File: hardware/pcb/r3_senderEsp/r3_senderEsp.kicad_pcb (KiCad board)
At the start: 2 copper layers, 165.5 x 125.5 mm, 17 parts, among them J1 RFID-RC522, J2 KY-021, J3 KY-021, J4 Links, J5 Rechts

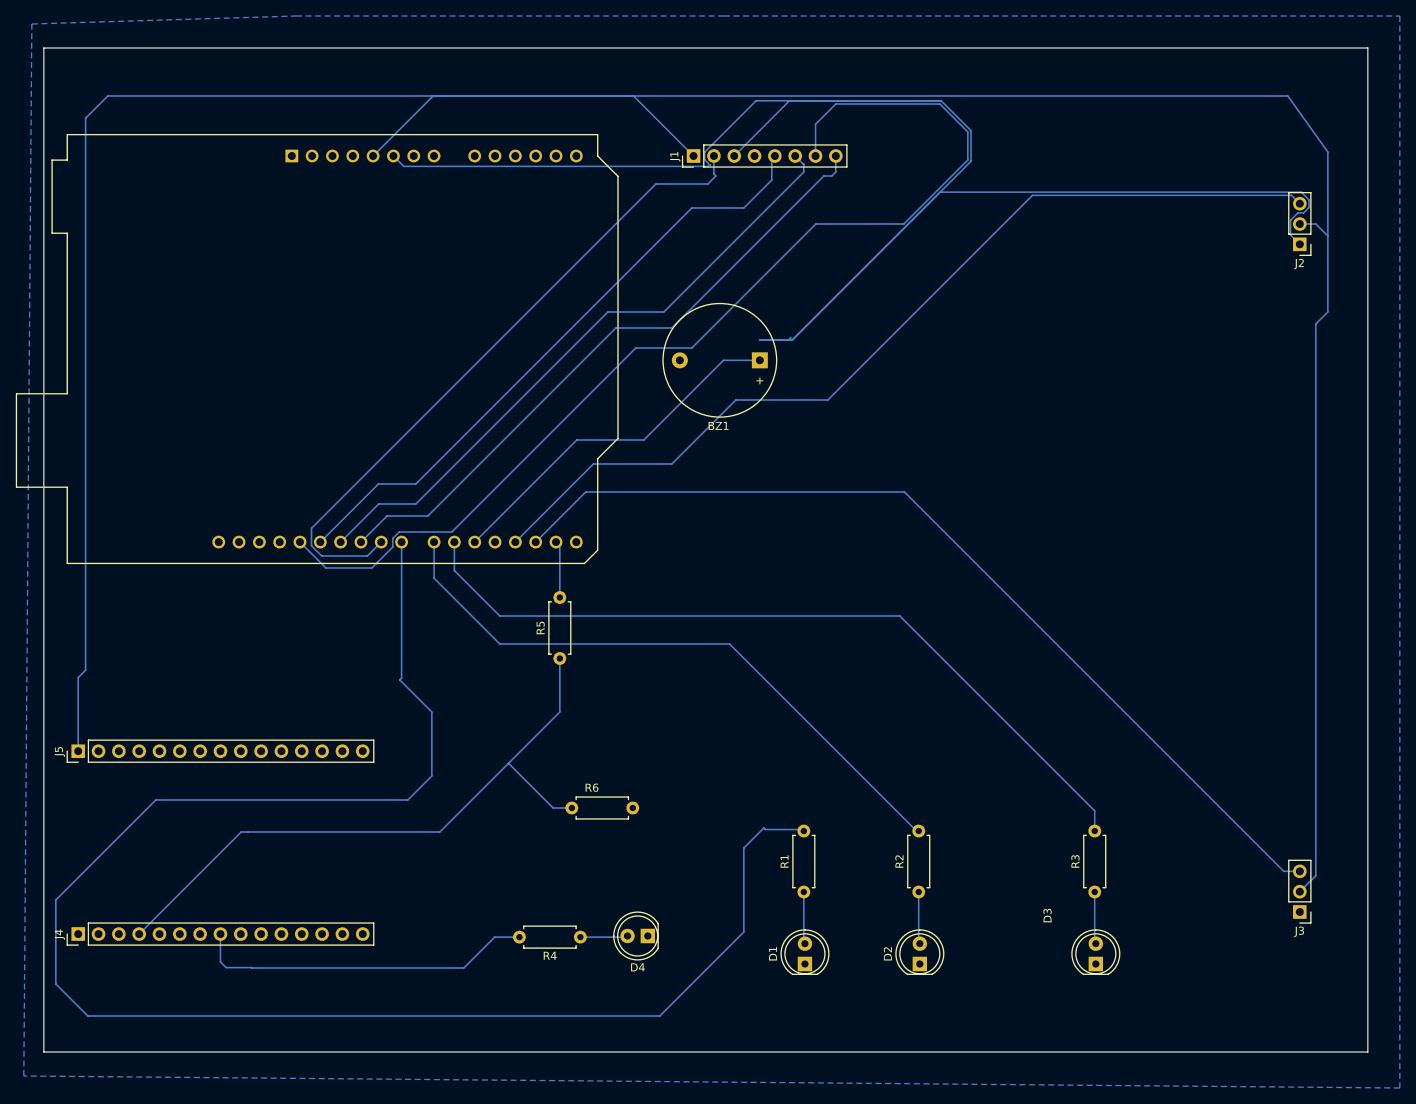
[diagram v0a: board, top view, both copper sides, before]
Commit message: Add files via upload
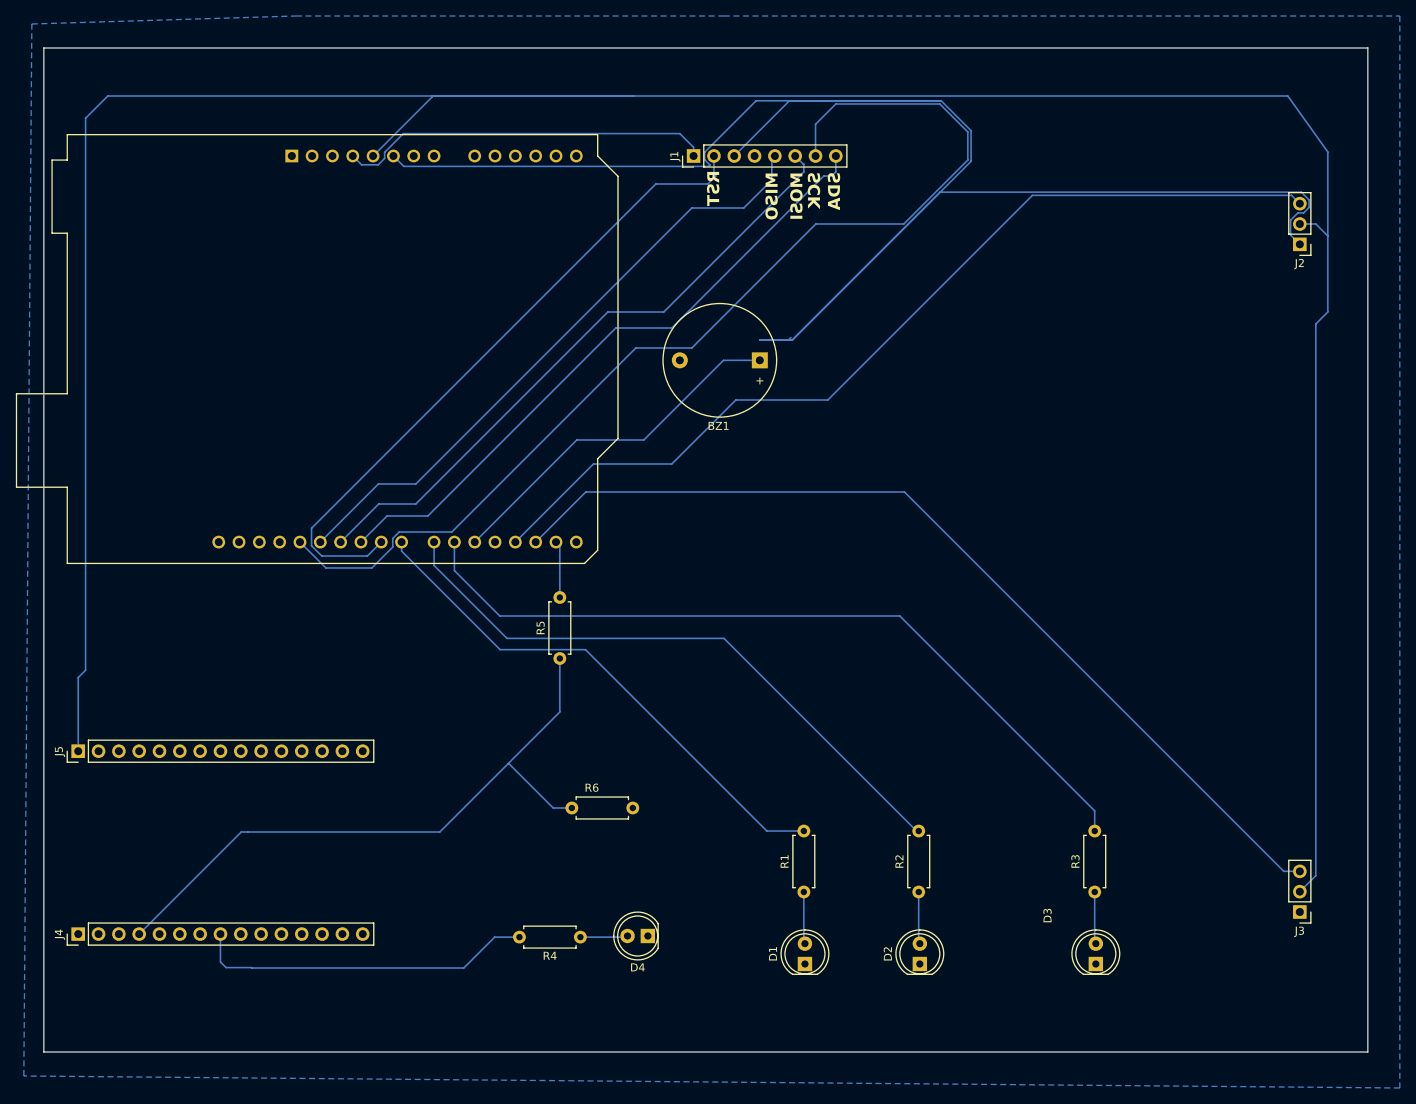
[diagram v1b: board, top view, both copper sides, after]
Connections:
- A1 pad 4: unconnected-(A1-3V3-Pad4) -> Net-(A1-3V3)
- J1 pad 1: +5V -> Net-(A1-3V3)
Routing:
- net Net-(A1-D8): track 206.0 -> 65.9 mm
- net Net-(A1-3V3): track 0.00 -> 46.9 mm
- net +5V: track 257.8 -> 247.2 mm
- net Net-(A1-D7): track 78.3 -> 77.4 mm
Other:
- board text added: "MISO"
- board text added: "MOSI"
- board text added: "RST"
- board text added: "SCK"
- board text added: "SDA"
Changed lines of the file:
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@@
 			(drillshape 0)
 			(scaleselection 1)
-			(outputdirectory "Kicad Datein/GerberBohrungen/")
+			(outputdirectory "r3_senderEsp_GerberBohrungen")
 		)
 	)
@@
 	(net 1 "Net-(A1-D2)")
 	(net 2 "unconnected-(A1-A2-Pad11)")
-	(net 3 "unconnected-(A1-3V3-Pad4)")
+	(net 3 "Net-(A1-3V3)")
 	(net 4 "Net-(A1-D13)")
 	(net 5 "unconnected-(A1-D0{slash}RX-Pad15)")
@@
 		(property ki_fp_filters "LED* LED_SMD:* LED_THT:*")
 		(sheetname "/")
-		(sheetfile "R3Sender.kicad_sch")
+		(sheetfile "r3_senderEsp.kicad_sch")
 		(attr through_hole)
 		(fp_line
@@
 		(property ki_fp_filters "Connector*:*_1x??_*")
 		(sheetname "/")
-		(sheetfile "R3Sender.kicad_sch")
+		(sheetfile "r3_senderEsp.kicad_sch")
 		(attr through_hole)
 		(fp_line
@@
 			(layers "*.Cu" "*.Mask")
 			(remove_unused_layers no)
-			(net 10 "+5V")
+			(net 3 "Net-(A1-3V3)")
 			(pinfunction "Pin_1")
 			(pintype "passive")
@@
 		(property ki_fp_filters "Connector*:*_1x??_*")
 		(sheetname "/")
-		(sheetfile "R3Sender.kicad_sch")
+		(sheetfile "r3_senderEsp.kicad_sch")
 		(attr through_hole)
 		(fp_line
@@
 		(property ki_fp_filters "R_*")
 		(sheetname "/")
-		(sheetfile "R3Sender.kicad_sch")
+		(sheetfile "r3_senderEsp.kicad_sch")
 		(attr through_hole)
 		(fp_line
@@
 		(property ki_fp_filters "R_*")
 		(sheetname "/")
-		(sheetfile "R3Sender.kicad_sch")
+		(sheetfile "r3_senderEsp.kicad_sch")
 		(attr through_hole)
 		(fp_line
@@
 		(property ki_fp_filters "Arduino*UNO*R3*")
 		(sheetname "/")
-		(sheetfile "R3Sender.kicad_sch")
+		(sheetfile "r3_senderEsp.kicad_sch")
 		(attr through_hole)
 		(fp_line
@@
 			(layers "*.Cu" "*.Mask")
 			(remove_unused_layers no)
-			(net 3 "unconnected-(A1-3V3-Pad4)")
+			(net 3 "Net-(A1-3V3)")
 			(pinfunction "3V3")
 			(pintype "power_out")
@@
 		(property ki_fp_filters "LED* LED_SMD:* LED_THT:*")
 		(sheetname "/")
-		(sheetfile "R3Sender.kicad_sch")
+		(sheetfile "r3_senderEsp.kicad_sch")
 		(attr through_hole)
 		(fp_line
@@
 		(property ki_fp_filters "LED* LED_SMD:* LED_THT:*")
 		(sheetname "/")
-		(sheetfile "R3Sender.kicad_sch")
+		(sheetfile "r3_senderEsp.kicad_sch")
 		(attr through_hole)
 		(fp_line
@@
 		(property ki_fp_filters "R_*")
 		(sheetname "/")
-		(sheetfile "R3Sender.kicad_sch")
+		(sheetfile "r3_senderEsp.kicad_sch")
 		(attr through_hole)
 		(fp_line
@@
 		(property ki_fp_filters "Connector*:*_1x??_*")
 		(sheetname "/")
-		(sheetfile "R3Sender.kicad_sch")
+		(sheetfile "r3_senderEsp.kicad_sch")
 		(attr through_hole)
 		(fp_line
@@
 		(property ki_fp_filters "R_*")
 		(sheetname "/")
-		(sheetfile "R3Sender.kicad_sch")
+		(sheetfile "r3_senderEsp.kicad_sch")
 		(attr through_hole)
 		(fp_line
@@
 		(property ki_fp_filters "LED* LED_SMD:* LED_THT:*")
 		(sheetname "/")
-		(sheetfile "R3Sender.kicad_sch")
+		(sheetfile "r3_senderEsp.kicad_sch")
 		(attr through_hole)
 		(fp_line
@@
 		(property ki_fp_filters "R_*")
 		(sheetname "/")
-		(sheetfile "R3Sender.kicad_sch")
+		(sheetfile "r3_senderEsp.kicad_sch")
 		(attr through_hole)
 		(fp_line
@@
 		(property ki_fp_filters "Connector*:*_1x??_*")
 		(sheetname "/")
-		(sheetfile "R3Sender.kicad_sch")
+		(sheetfile "r3_senderEsp.kicad_sch")
 		(attr through_hole)
 		(fp_line
@@
 		(property ki_fp_filters "*Buzzer*")
 		(sheetname "/")
-		(sheetfile "R3Sender.kicad_sch")
+		(sheetfile "r3_senderEsp.kicad_sch")
 		(attr through_hole)
 		(fp_circle
@@
 		(property ki_fp_filters "Connector*:*_1x??_*")
 		(sheetname "/")
-		(sheetfile "R3Sender.kicad_sch")
+		(sheetfile "r3_senderEsp.kicad_sch")
 		(attr through_hole)
 		(fp_line
@@
 		(property ki_fp_filters "R_*")
 		(sheetname "/")
-		(sheetfile "R3Sender.kicad_sch")
+		(sheetfile "r3_senderEsp.kicad_sch")
 		(attr through_hole)
 		(fp_line
@@
 		(layer "Edge.Cuts")
 	)
+	(gr_text "MISO"
+		(at 110.4 24 90)
+		(layer "F.SilkS")
+		(effects
+			(font
+				(size 1.5 1.5)
+				(thickness 0.3)
+				(bold yes)
+			)
+			(justify left bottom mirror)
+		)
+	)
+	(gr_text "SCK"
+		(at 115.7 24 90)
+		(layer "F.SilkS")
+		(effects
+			(font
+				(size 1.5 1.5)
+				(thickness 0.3)
+				(bold yes)
+			)
+			(justify left bottom mirror)
+		)
+	)
+	(gr_text "RST"
+		(at 103.1 23.8 90)
+		(layer "F.SilkS")
+		(effects
+			(font
+				(size 1.5 1.5)
+				(thickness 0.3)
+				(bold yes)
+			)
+			(justify left bottom mirror)
+		)
+	)
+	(gr_text "MOSI"
+		(at 113.5 24 90)
+		(layer "F.SilkS")
+		(effects
+			(font
+				(size 1.5 1.5)
+				(thickness 0.3)
+				(bold yes)
+			)
+			(justify left bottom mirror)
+		)
+	)
+	(gr_text "SDA"
+		(at 118.2 24 90)
+		(layer "F.SilkS")
+		(effects
+			(font
+				(size 1.5 1.5)
+				(thickness 0.3)
+				(bold yes)
+			)
+			(justify left bottom mirror)
+		)
+	)
 	(segment
 		(start 79.98 70.26)
@@
 	)
 	(segment
+		(start 61.099 21.54395)
+		(end 63.44295 19.2)
+		(width 0.2)
+		(layer "B.Cu")
+		(net 3)
+	)
+	(segment
+		(start 57.12 22)
+		(end 58.221 23.101)
+		(width 0.2)
+		(layer "B.Cu")
+		(net 3)
+	)
+	(segment
+		(start 99.72 20.92)
+		(end 99.72 22)
+		(width 0.2)
+		(layer "B.Cu")
+		(net 3)
+	)
+	(segment
+		(start 98 19.2)
+		(end 99.72 20.92)
+		(width 0.2)
+		(layer "B.Cu")
+		(net 3)
+	)
+	(segment
+		(start 63.44295 19.2)
+		(end 98 19.2)
+		(width 0.2)
+		(layer "B.Cu")
+		(net 3)
+	)
+	(segment
+		(start 60.299 23.101)
+		(end 61.099 22.301)
+		(width 0.2)
+		(layer "B.Cu")
+		(net 3)
+	)
+	(segment
+		(start 61.099 22.301)
+		(end 61.099 21.54395)
+		(width 0.2)
+		(layer "B.Cu")
+		(net 3)
+	)
+	(segment
+		(start 58.221 23.101)
+		(end 60.299 23.101)
+		(width 0.2)
+		(layer "B.Cu")
+		(net 3)
+	)
+	(segment
 		(start 62.119 69.80395)
 		(end 62.92295 69)
@@
 	)
 	(segment
-		(start 63.22 70.26)
-		(end 63.22 87.28)
+		(start 86.209 83.709)
+		(end 75.53763 83.709)
 		(width 0.2)
 		(layer "B.Cu")
@@
 	)
 	(segment
-		(start 108.69 106.19)
-		(end 113.5 106.19)
+		(start 75.53763 83.709)
+		(end 63.22 71.39137)
 		(width 0.2)
 		(layer "B.Cu")
@@
 	)
 	(segment
-		(start 106 108.5)
-		(end 108.5 106)
+		(start 63.22 71.39137)
+		(end 63.22 70.26)
 		(width 0.2)
 		(layer "B.Cu")
@@
 	)
 	(segment
-		(start 108.5 106)
-		(end 108.69 106.19)
+		(start 113.5 106.38)
+		(end 108.88 106.38)
 		(width 0.2)
 		(layer "B.Cu")
@@
 	)
 	(segment
-		(start 64 102.5)
-		(end 32.5 102.5)
-		(width 0.2)
-		(layer "B.Cu")
-		(net 6)
-	)
-	(segment
-		(start 67 99.5)
-		(end 64 102.5)
-		(width 0.2)
-		(layer "B.Cu")
-		(net 6)
-	)
-	(segment
-		(start 95.5 129.5)
-		(end 106 119)
-		(width 0.2)
-		(layer "B.Cu")
-		(net 6)
-	)
-	(segment
-		(start 63.22 87.28)
-		(end 63 87.5)
-		(width 0.2)
-		(layer "B.Cu")
-		(net 6)
-	)
-	(segment
-		(start 20 125.5)
-		(end 24 129.5)
-		(width 0.2)
-		(layer "B.Cu")
-		(net 6)
-	)
-	(segment
-		(start 32.5 102.5)
-		(end 20 115)
-		(width 0.2)
-		(layer "B.Cu")
-		(net 6)
-	)
-	(segment
-		(start 67 91.5)
-		(end 67 99.5)
-		(width 0.2)
-		(layer "B.Cu")
-		(net 6)
-	)
-	(segment
-		(start 106 119)
-		(end 106 108.5)
-		(width 0.2)
-		(layer "B.Cu")
-		(net 6)
-	)
-	(segment
-		(start 24 129.5)
-		(end 95.5 129.5)
-		(width 0.2)
-		(layer "B.Cu")
-		(net 6)
-	)
-	(segment
-		(start 63 87.5)
-		(end 67 91.5)
-		(width 0.2)
-		(layer "B.Cu")
-		(net 6)
-	)
-	(segment
-		(start 20 115)
-		(end 20 125.5)
+		(start 108.88 106.38)
+		(end 86.209 83.709)
 		(width 0.2)
 		(layer "B.Cu")
@@
 	)
 	(segment
-		(start 99.72 22)
-		(end 92.22 14.5)
-		(width 0.2)
-		(layer "B.Cu")
-		(net 10)
-	)
-	(segment
 		(start 179 32)
 		(end 177.5 30.5)
@@
 	)
 	(segment
-		(start 67.28 70.26)
-		(end 67.28 74.78)
+		(start 76.4 82.3)
+		(end 103.52 82.3)
 		(width 0.2)
 		(layer "B.Cu")
@@
 	)
 	(segment
-		(start 75.5 83)
-		(end 104.22 83)
+		(start 67.28 70.26)
+		(end 67.28 73.18)
 		(width 0.2)
 		(layer "B.Cu")
@@
 	)
 	(segment
-		(start 104.22 83)
+		(start 103.52 82.3)
 		(end 127.86 106.64)
 		(width 0.2)
@@
 	)
 	(segment
-		(start 67.28 74.78)
-		(end 75.5 83)
+		(start 67.28 73.18)
+		(end 76.4 82.3)
 		(width 0.2)
 		(layer "B.Cu")
